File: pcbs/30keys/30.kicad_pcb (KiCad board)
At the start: 2 copper layers, 116.9 x 79.4 mm, 20 parts, among them SW1 SW_PUSH, SW10 SW_PUSH, SW11 SW_PUSH, SW12 SW_PUSH, SW13 SW_PUSH, SW14 SW_PUSH, SW15 SW_PUSH, SW2 SW_PUSH, SW3 SW_PUSH, SW4 SW_PUSH, SW5 SW_PUSH, SW6 SW_PUSH, SW7 SW_PUSH, SW8 SW_PUSH, SW9 SW_PUSH, U1 ProMicro

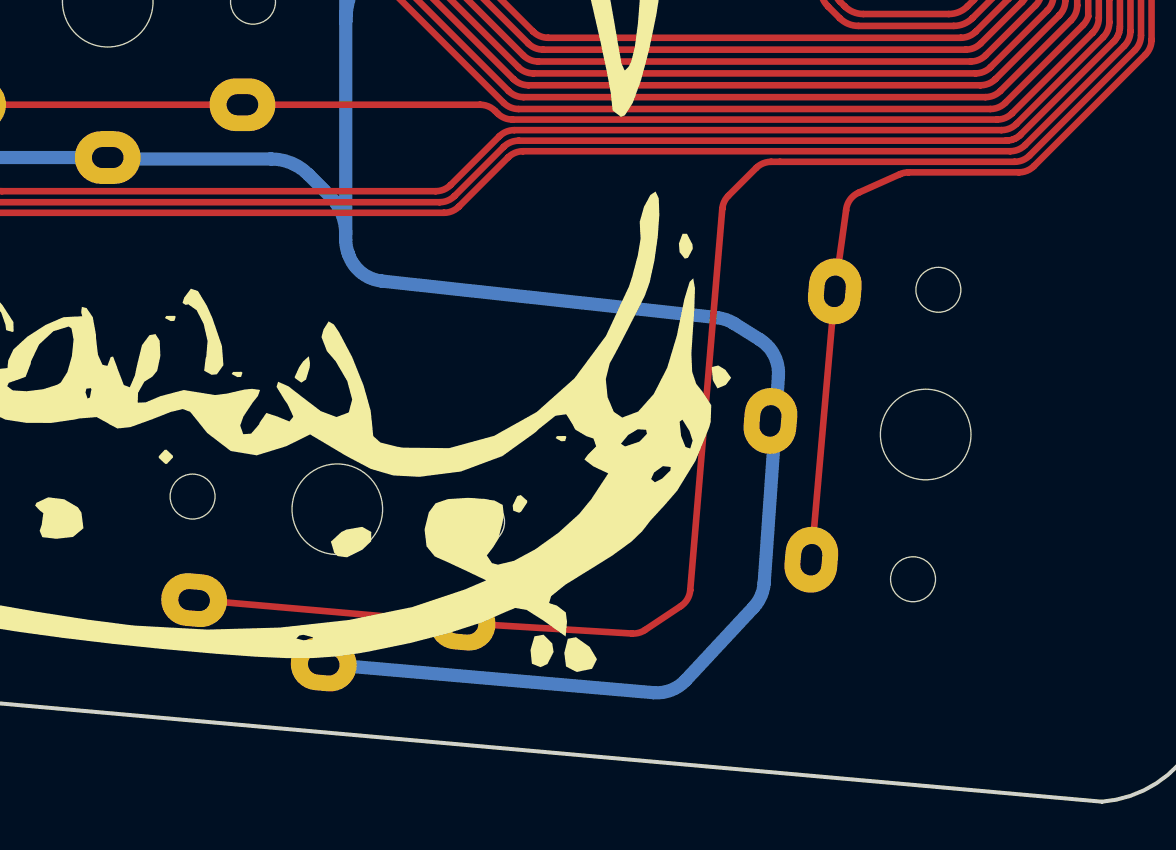
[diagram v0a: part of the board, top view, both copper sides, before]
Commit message: thumb alignment
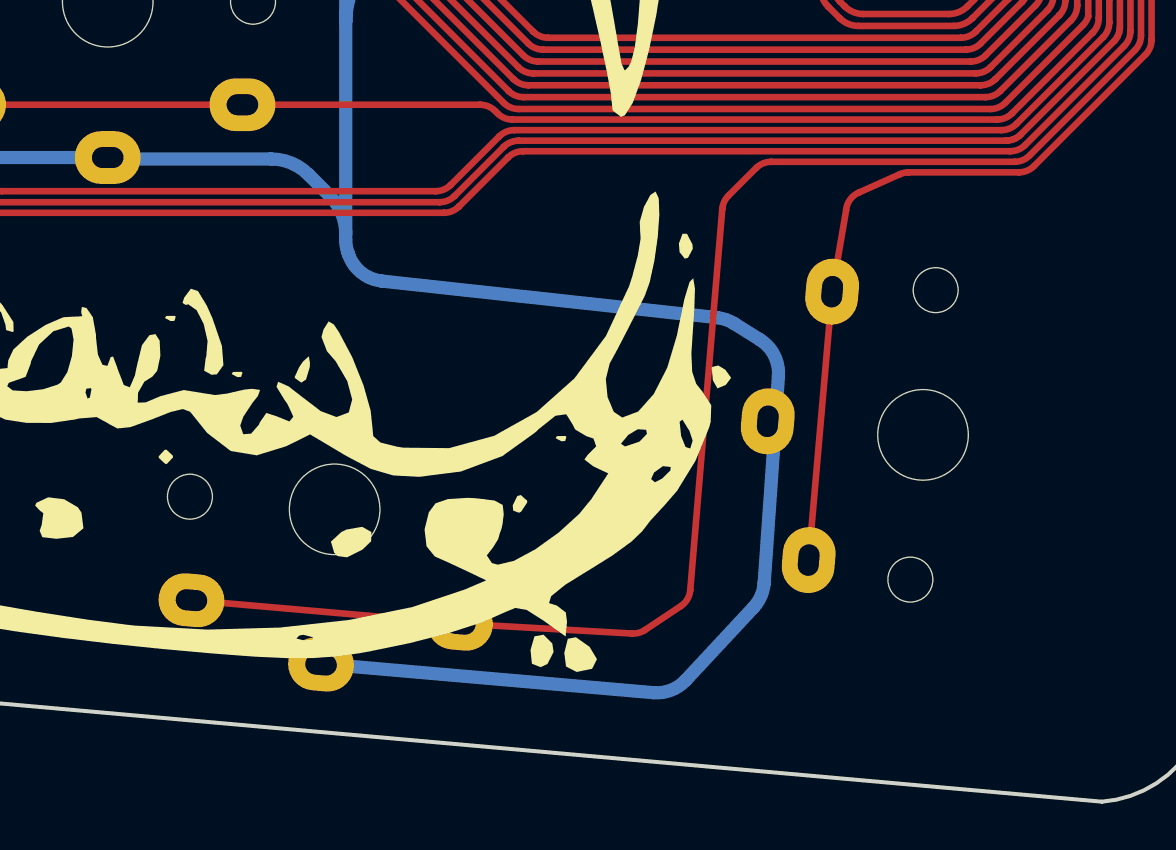
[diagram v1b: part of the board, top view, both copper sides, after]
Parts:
- moved SW15 0.10 mm to (128.1, 110.8)
- moved SW14 0.10 mm to (105.8, 113.6)
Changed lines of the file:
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@@
       (drillshape 0)
       (scaleselection 1)
-      (outputdirectory "/home/doyle/keeborbs/gerbers/30/")
+      (outputdirectory "/home/doyle/keyboards/gerbers/30keys/")
     )
   )
@@
   )
   (footprint "bugs:Choc_reversible_15u" (layer "F.Cu")
-    (at 105.924464 113.641751 -5)
+    (at 105.823864 113.646178 -5)
     (descr "Kailh \"Choc\" PG1350 keyswitch")
     (tags "kailh,choc")
@@
     (property "Sheetname" "")
     (attr through_hole)
-    (fp_text reference "SW14" (at 0 3 -5) (layer "F.SilkS") hide
+    (fp_text reference "SW14" (at 0 3 175) (layer "F.SilkS") hide
       (effects (font (size 1 1) (thickness 0.15)))
     )
-    (fp_text value "SW_PUSH" (at 0 -5.5 -5) (layer "Cmts.User") hide
+    (fp_text value "SW_PUSH" (at 0 -5.5 175) (layer "Cmts.User") hide
       (effects (font (size 1 1) (thickness 0.15)))
     )
@@
   )
   (footprint "bugs:Choc_reversible_15u" (layer "F.Cu")
-    (at 128.199608 110.813279 -95)
+    (at 128.09823 110.826597 -95)
     (descr "Kailh \"Choc\" PG1350 keyswitch")
     (tags "kailh,choc")
@@
     (property "Sheetname" "")
     (attr through_hole)
-    (fp_text reference "SW15" (at 0 3 -95) (layer "F.SilkS") hide
+    (fp_text reference "SW15" (at 0 3 85) (layer "F.SilkS") hide
       (effects (font (size 1 1) (thickness 0.15)))
     )
-    (fp_text value "SW_PUSH" (at 0 -5.5 -95) (layer "Cmts.User") hide
+    (fp_text value "SW_PUSH" (at 0 -5.5 85) (layer "Cmts.User") hide
       (effects (font (size 1 1) (thickness 0.15)))
     )
@@
   (segment (start 137.965007 78.939446) (end 130.155115 78.939445) (width 0.25) (layer "B.Cu") (net 14))
   (arc (start 129.801563 79.08589) (mid 129.963774 78.977505) (end 130.155115 78.939445) (width 0.25) (layer "B.Cu") (net 14))
-  (segment (start 122.682 100.48816) (end 122.347211 100.48816) (width 0.25) (layer "F.Cu") (net 15))
-  (segment (start 136.116765 96.267259) (end 132.130178 100.253846) (width 0.25) (layer "F.Cu") (net 15))
-  (segment (start 117.079459 118.347644) (end 110.760658 117.962786) (width 0.25) (layer "F.Cu") (net 15))
-  (segment (start 120.498487 102.272702) (end 119.285317 116.709426) (width 0.25) (layer "F.Cu") (net 15))
-  (segment (start 138.965009 89.734442) (end 138.807116 89.734443) (width 0.25) (layer "F.Cu") (net 15))
-  (segment (start 137.965007 89.099443) (end 136.585395 90.479055) (width 0.25) (layer "F.Cu") (net 15))
-  (segment (start 136.351081 91.04474) (end 136.35108 95.701573) (width 0.25) (layer "F.Cu") (net 15))
   (segment (start 118.931887 117.308075) (end 117.571854 118.214764) (width 0.25) (layer "F.Cu") (net 15))
-  (segment (start 138.453559 89.587996) (end 137.965007 89.099443) (width 0.25) (layer "F.Cu") (net 15))
+  (segment (start 137.965007 89.099443) (end 136.585395 90.479055) (width 0.25) (layer "F.Cu") (net 15))
+  (segment (start 138.965009 89.734442) (end 138.807116 89.734443) (width 0.25) (layer "F.Cu") (net 15))
+  (segment (start 131.564493 100.48816) (end 122.347211 100.48816) (width 0.25) (layer "F.Cu") (net 15))
   (segment (start 121.781525 100.722475) (end 120.729992 101.774008) (width 0.25) (layer "F.Cu") (net 15))
-  (segment (start 110.760658 117.962786) (end 100.599472 117.073797) (width 0.25) (layer "F.Cu") (net 15))
-  (segment (start 131.564493 100.48816) (end 122.682 100.48816) (width 0.25) (layer "F.Cu") (net 15))
+  (segment (start 138.453559 89.587996) (end 137.965007 89.099443) (width 0.25) (layer "F.Cu") (net 15))
+  (segment (start 110.56455 117.975832) (end 100.403364 117.086843) (width 0.25) (layer "F.Cu") (net 15))
+  (segment (start 120.498487 102.272702) (end 119.285317 116.709426) (width 0.25) (layer "F.Cu") (net 15))
+  (segment (start 136.116765 96.267259) (end 132.130178 100.253846) (width 0.25) (layer "F.Cu") (net 15))
+  (segment (start 117.079459 118.347644) (end 110.56455 117.975832) (width 0.25) (layer "F.Cu") (net 15))
+  (segment (start 136.351081 91.04474) (end 136.35108 95.701573) (width 0.25) (layer "F.Cu") (net 15))
   (via (at 137.965007 89.099443) (size 0.8) (drill 0.4) (layers "F.Cu" "B.Cu") (net 15))
-  (arc (start 118.931887 117.308075) (mid 119.177028 117.049148) (end 119.285317 116.709426) (width 0.25) (layer "F.Cu") (net 15))
+  (arc (start 117.571854 118.214764) (mid 117.336529 118.321493) (end 117.079459 118.347644) (width 0.25) (layer "F.Cu") (net 15))
+  (arc (start 132.130178 100.253846) (mid 131.870639 100.427264) (end 131.564493 100.48816) (width 0.25) (layer "F.Cu") (net 15))
   (arc (start 138.807116 89.734443) (mid 138.615772 89.696383) (end 138.453559 89.587996) (width 0.25) (layer "F.Cu") (net 15))
-  (arc (start 122.347211 100.48816) (mid 122.041064 100.549057) (end 121.781525 100.722475) (width 0.25) (layer "F.Cu") (net 15))
   (arc (start 120.729992 101.774008) (mid 120.570053 102.002842) (end 120.498487 102.272702) (width 0.25) (layer "F.Cu") (net 15))
-  (arc (start 136.585395 90.479055) (mid 136.411977 90.738594) (end 136.351081 91.04474) (width 0.25) (layer "F.Cu") (net 15))
-  (arc (start 117.079459 118.347644) (mid 117.336529 118.321493) (end 117.571854 118.214764) (width 0.25) (layer "F.Cu") (net 15))
   (arc (start 136.35108 95.701573) (mid 136.290184 96.00772) (end 136.116765 96.267259) (width 0.25) (layer "F.Cu") (net 15))
-  (arc (start 132.130178 100.253846) (mid 131.870639 100.427264) (end 131.564493 100.48816) (width 0.25) (layer "F.Cu") (net 15))
+  (arc (start 136.585395 90.479055) (mid 136.411977 90.738594) (end 136.351081 91.04474) (width 0.25) (layer "F.Cu") (net 15))
+  (arc (start 122.347211 100.48816) (mid 122.041064 100.549057) (end 121.781525 100.722475) (width 0.25) (layer "F.Cu") (net 15))
+  (arc (start 119.285317 116.709426) (mid 119.177028 117.049148) (end 118.931887 117.308075) (width 0.25) (layer "F.Cu") (net 15))
   (segment (start 137.965007 89.099443) (end 130.155115 89.099445) (width 0.25) (layer "B.Cu") (net 15))
   (segment (start 129.801562 89.245891) (end 129.313009 89.734443) (width 0.25) (layer "B.Cu") (net 15))
   (arc (start 130.155115 89.099445) (mid 129.963774 89.137505) (end 129.801562 89.245891) (width 0.25) (layer "B.Cu") (net 15))
-  (segment (start 124.758943 105.392779) (end 125.185656 102.328647) (width 0.25) (layer "F.Cu") (net 16))
-  (segment (start 123.869954 115.553965) (end 124.758943 105.392779) (width 0.25) (layer "F.Cu") (net 16))
+  (segment (start 125.185656 102.328647) (end 124.657565 105.406097) (width 0.25) (layer "F.Cu") (net 16))
   (segment (start 138.833817 92.274446) (end 138.965006 92.274446) (width 0.25) (layer "F.Cu") (net 16))
   (segment (start 137.668 91.694) (end 136.984915 92.377085) (width 0.25) (layer "F.Cu") (net 16))
   (segment (start 137.922 91.694) (end 137.668 91.694) (width 0.25) (layer "F.Cu") (net 16))
   (segment (start 127.225044 100.957482) (end 125.656501 101.659527) (width 0.25) (layer "F.Cu") (net 16))
+  (segment (start 123.768576 115.567283) (end 124.657565 105.406097) (width 0.25) (layer "F.Cu") (net 16))
   (segment (start 136.516286 96.432744) (end 132.295664 100.653366) (width 0.25) (layer "F.Cu") (net 16))
   (segment (start 136.750601 92.94277) (end 136.750601 95.867058) (width 0.25) (layer "F.Cu") (net 16))
